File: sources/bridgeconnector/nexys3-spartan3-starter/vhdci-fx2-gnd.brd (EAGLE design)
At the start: 44.1 x 76.2 mm, 9 parts, among them X1 CLK, X2 TRIGGER

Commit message: bla
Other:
- board text added: "/home/jkaps/public_html/cerg/design/CERG-logo-with-url-bw.bmp"
- board text added: "1"
- board text added: "2"
- board text added: "49"
- board text added: "50"
- board text added: "A"
- board text added: "Alternate DUT"
- board text added: "B"
- board text added: "CLK"
- board text added: "CLK_C2D"
- board text added: "CLK_E2C"
- board text added: "CLK_E2D"
- board text added: "Control"
- board text added: "DUT"
- board text added: "JP1"
- board text added: "JP2"
- board text added: "JP3"
- board text added: "JP4"
- board text added: "JP5"
- board text added: "TRIGGER"
- board text added: "TRIGGER_2D"
- board text added: "X1"
- board text added: "X2"

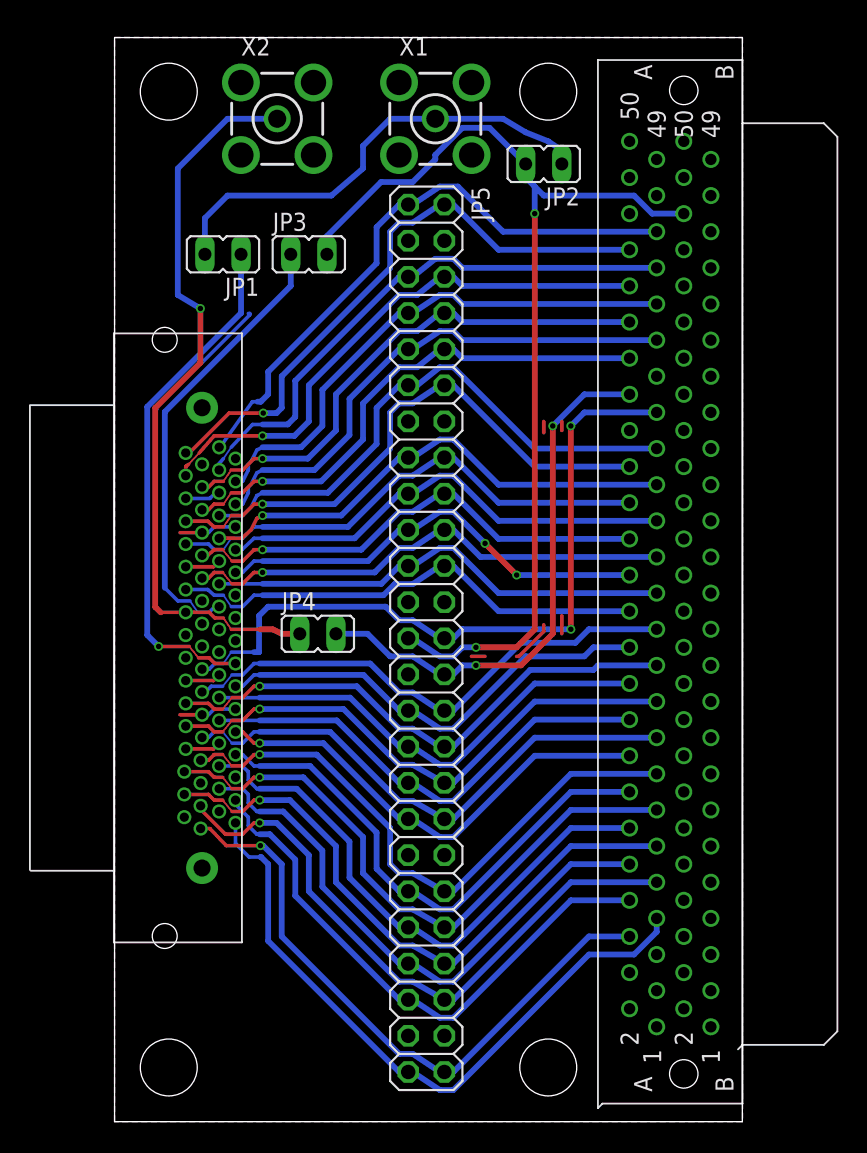
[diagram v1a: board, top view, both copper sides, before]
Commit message: bla
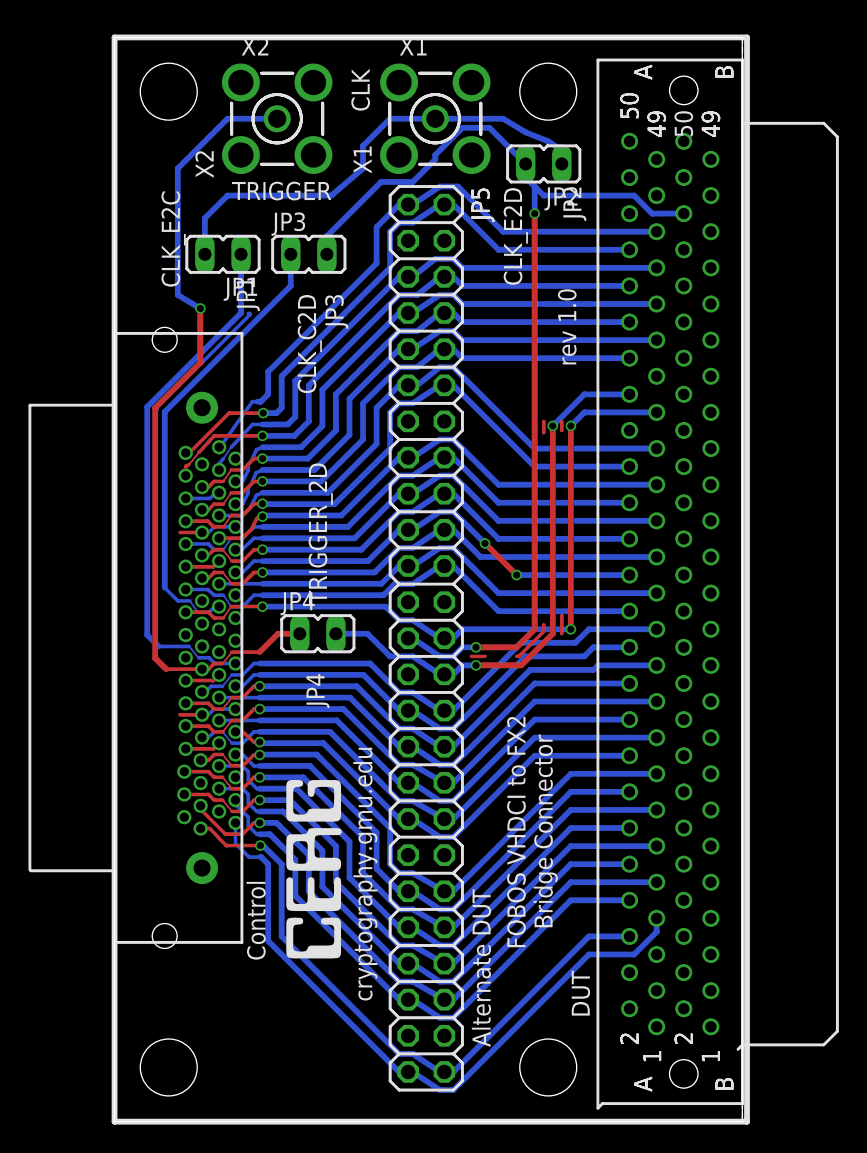
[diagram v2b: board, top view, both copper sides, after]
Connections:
- net RST: now also U$2.V49; no longer U$2.V54
- net TRIGGER: now also U$2.V54; no longer U$2.V49
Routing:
- net TRIGGER: track 52.4 -> 56.6 mm
- net RST: track 51.1 -> 49.4 mm, vias 2 -> 3
- net CLKIN_C: vias 1 -> 0
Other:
- board text added: "FOBOS VHDCI to FX2 Bridge Connector"
- board text added: "cryptography.gmu.edu"
- board text added: "rev 1.0"
